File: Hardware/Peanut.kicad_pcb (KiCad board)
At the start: 2 copper layers, 96.8 x 57 mm, 54 parts, among them J1 Conn_02x04_Odd_Even, J2 Conn_02x04_Odd_Even, J3 AudioPlug3, SW1 Push_Button, SW2 Push_Button, SW3 Push_Button, SW4 Push_Button, SW5 Slide Switch, SW6 Slide Switch, U1 BNO085, U2 PCF8574, U3 HDC2010YPAR, U4 LTR-303ALS-01, U5 MCP4728T-E/UN, U6 LWP040-PSGLC-S, Y1 Crystal_32.768kHz

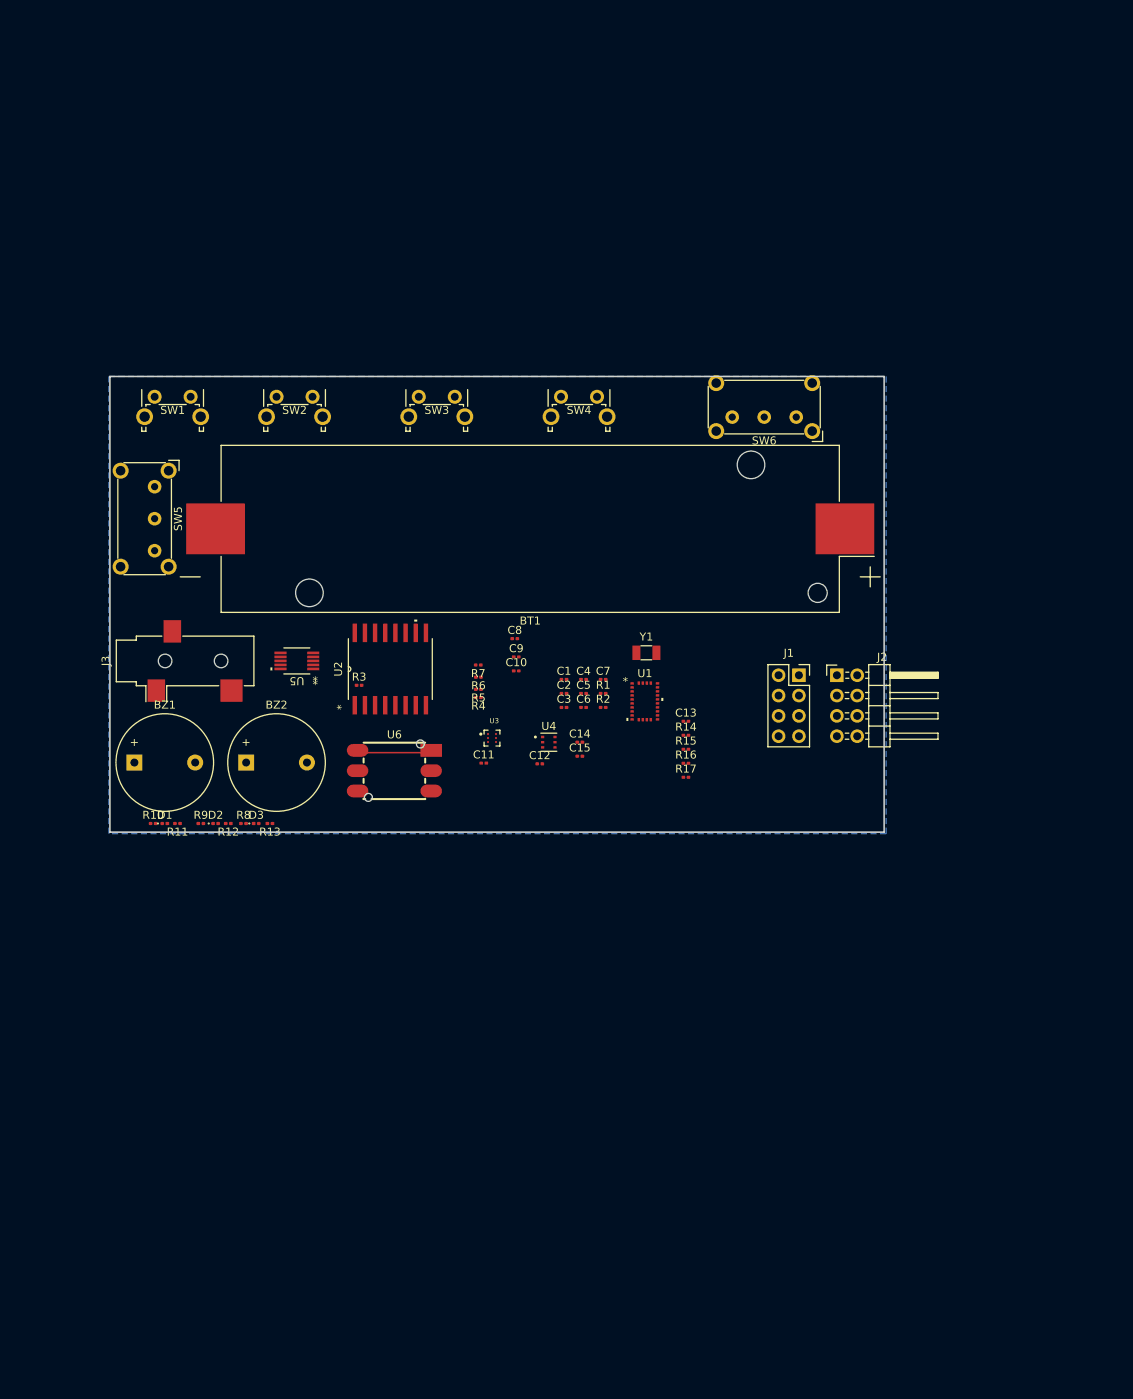
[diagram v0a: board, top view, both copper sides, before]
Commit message: Fully wired board!
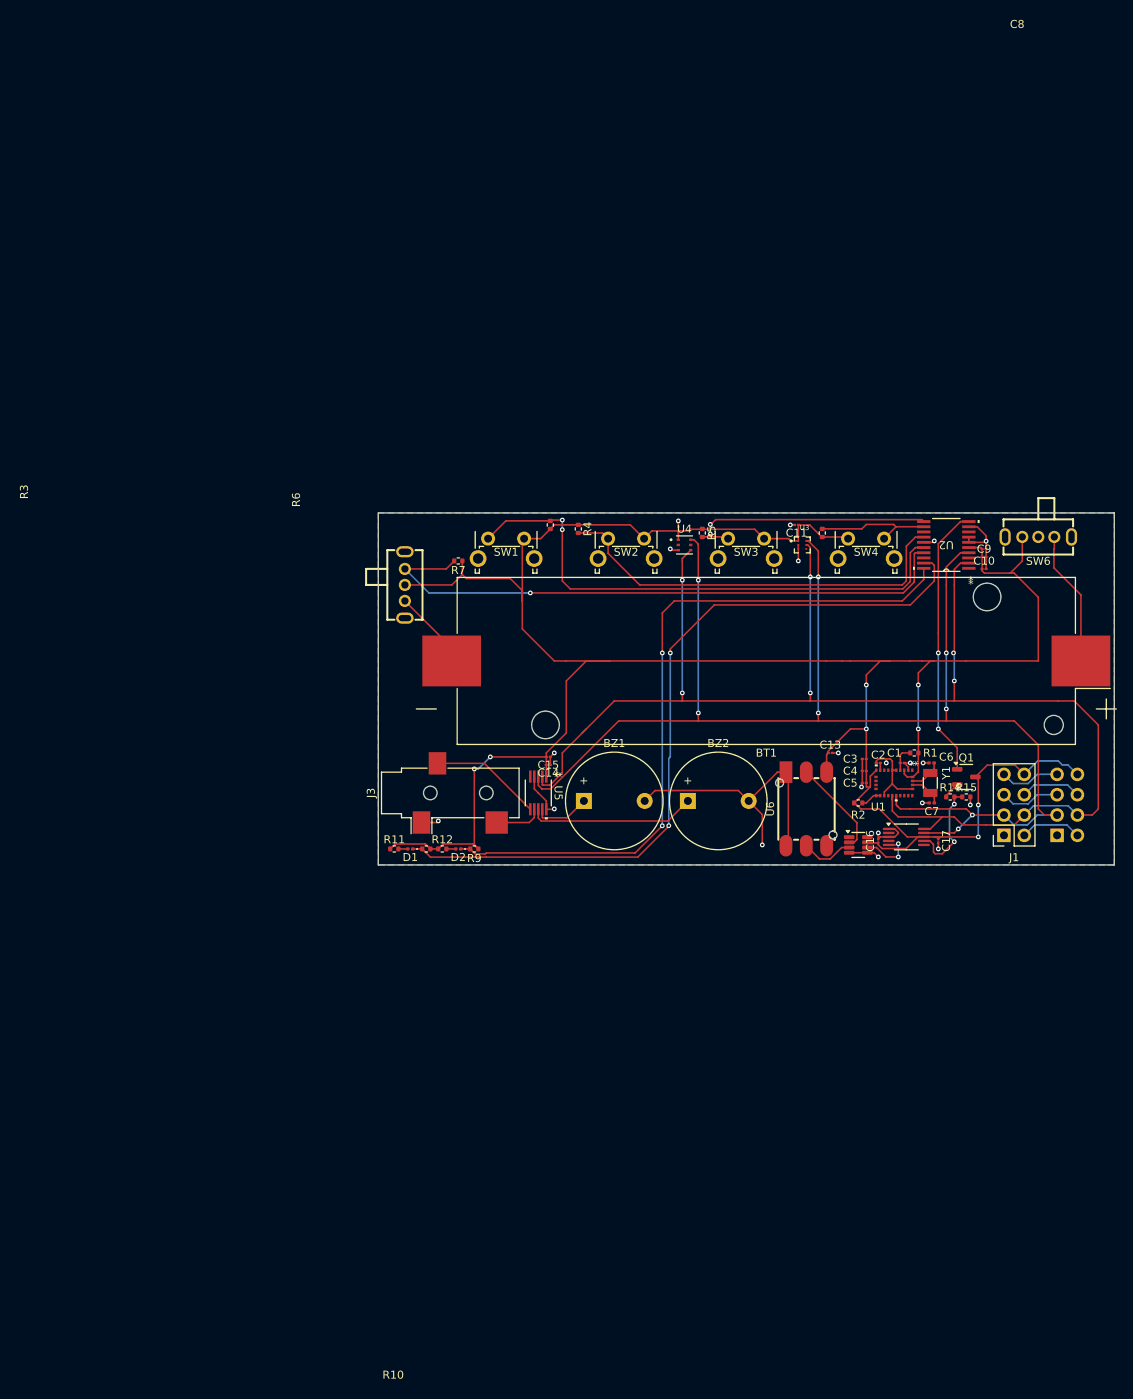
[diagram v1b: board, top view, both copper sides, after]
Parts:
- removed D3: BLU, LED_SMD:LED_0201_0603Metric
- removed R13: 2.2k, Resistor_SMD:R_0201_0603Metric
- removed R16, R17: 56k, Resistor_SMD:R_0201_0603Metric
- removed R8: 100k, Resistor_SMD:R_0201_0603Metric
- added C16: 0.1uF, Resistor_SMD:R_01005_0402Metric, F.Cu at (156.5, 86.0)
- added C17: 0.1uF, Resistor_SMD:R_01005_0402Metric, F.Cu at (164.0, 86.0)
- added Q1: Q_NPN_BEC, Package_TO_SOT_SMD:SOT-23-3, F.Cu at (167.5, 78.0)
- added U7: ADS1015IDGSR, Package_SO:VSSOP-10_3x3mm_P0.5mm, F.Cu at (160.0, 85.5)
- added U8: INA350ABSIDDFR, Package_TO_SOT_SMD:TSOT-23-8, F.Cu at (154.0, 86.5)
- C1, C10, C11, C12, C14, C15, C2, C3, C4, C5, C8, C9: footprint Capacitor_SMD:C_0201_0603Metric -> Resistor_SMD:R_01005_0402Metric
- C13: value 0.1uF -> 1uF; footprint Capacitor_SMD:C_0201_0603Metric -> Resistor_SMD:R_01005_0402Metric
- J2: footprint Connector_PinHeader_2.54mm:PinHeader_2x04_P2.54mm_Horizontal -> Peanut:PinHeader_2x04_P2.54mm_Horizontal_Flipped; moved to B.Cu
- R1, R10, R11, R12, R2, R3, R4, R5, R6, R7, R9: footprint Resistor_SMD:R_0201_0603Metric -> Resistor_SMD:R_0402_1005Metric
- R14, R15: value 1k -> R; footprint Resistor_SMD:R_0201_0603Metric -> Resistor_SMD:R_0402_1005Metric
- SW5, SW6: footprint Button_Switch_THT:SW_E-Switch_EG1224_SPDT_Angled -> Peanut:SW-TH_SK12D07VG4
- U2: value PCF8574 -> PCF8574APWR; footprint Peanut:DW16 -> Peanut:PW20
- moved U2 71.2 mm to (165.0, 49.0), turned to 180 degrees
- moved C10 59.8 mm to (169.7, 52.0)
- moved C9 59.8 mm to (169.7, 50.5)
- moved C8 59.7 mm to (169.7, 49.5)
- moved BZ1 56.4 mm to (119.7, 81.0)
- moved BZ2 55.4 mm to (132.7, 81.0)
- moved U6 51.7 mm to (147.5, 82.0), turned to 90 degrees
- moved C11 49.1 mm to (146.3, 46.5), turned to 180 degrees
- moved R6 46.6 mm to (149.5, 47.5), turned to 90 degrees
- moved U3 45.7 mm to (147.0, 49.0)
- moved SW1 45.3 mm to (107.7, 48.2)
- moved SW2 45.1 mm to (122.7, 48.2)
- moved C6 44.0 mm to (163.2, 76.2), turned to 180 degrees
- moved C7 43.9 mm to (163.2, 81.2), turned to 180 degrees
- moved C1 43.6 mm to (159.5, 76.2)
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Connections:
- C13 pad 1: GND -> +3V3
- C13 pad 2: /Pressure and ADC/PRESSURE -> GND
- R14 pad 1: Net-(U6-VOUT+) -> Net-(Q1-E)
- R14 pad 2: Net-(U7--) -> Net-(U7-AIN3)
- R15 pad 1: Net-(U7-+) -> Net-(U7-AIN3)
- R15 pad 2: Net-(U6-VOUT-) -> GND
- R3 pad 2: Net-(U2-P3) -> Net-(U2-P4)
- R4 pad 2: Net-(U2-P4) -> Net-(U2-P3)
- R5 pad 2: Net-(U2-P5) -> Net-(U2-P1)
- R6 pad 2: Net-(U2-P6) -> Net-(U2-P2)
- R7 pad 2: Net-(U2-P7) -> Net-(U2-P5)
- SW1 pad 1: Net-(U2-P3) -> Net-(U2-P4)
- SW2 pad 1: Net-(U2-P4) -> Net-(U2-P3)
- SW3 pad 1: Net-(U2-P5) -> Net-(U2-P1)
- SW4 pad 1: Net-(U2-P6) -> +3V3
- SW4 pad 2: +3V3 -> Net-(U2-P2)
- SW5 pad 1: Net-(U2-P7) -> Net-(U2-P5)
- U1 pad 17: /Motion Sensor/I2CADDR -> GND
- U2 pad 1: GND -> /DigitalMuxer/~{INT}
- U2 pad 10: Net-(U2-P5) -> /DigitalMuxer/P2
- U2 pad 11: Net-(U2-P6) -> Net-(U2-P1)
- U2 pad 12: Net-(U2-P7) -> Net-(U2-P2)
- U2 pad 13: /DigitalMuxer/Reset pin -> unconnected-(U2-NC-Pad13)
- U2 pad 14: SCL -> Net-(U2-P3)
- U2 pad 15: SDA -> GND
- U2 pad 16: +3V3 -> Net-(U2-P4)
- U2 pad 2: GND -> SCL
- U2 pad 3: GND -> unconnected-(U2-NC-Pad3)
- U2 pad 4: Net-(D1-K) -> SDA
- U2 pad 5: Net-(D2-K) -> +3V3
- U2 pad 6: Net-(D3-K) -> GND
- U2 pad 7: Net-(U2-P3) -> GND
- U2 pad 8: GND -> unconnected-(U2-NC-Pad8)
- U2 pad 9: Net-(U2-P4) -> GND
- U5 pad 5: unconnected-(U5-RDY/~{BSY}-Pad5) -> /DAC and Sound/RDY/~{BSY}
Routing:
- net +3V3: track 0.00 -> 320.3 mm, vias 0 -> 8
- net SCL: track 0.00 -> 180.2 mm, vias 0 -> 6
- net SDA: track 0.00 -> 179.0 mm, vias 0 -> 8
- net Net-(D1-K): track 0.00 -> 96.1 mm, vias 0 -> 2
- net GND: track 9.63 -> 100.2 mm, vias 0 -> 20
- net Net-(D2-K): track 0.00 -> 89.3 mm, vias 0 -> 2
- net Net-(U2-P5): track 0.00 -> 76.8 mm, vias 0 -> 1
- net Net-(U2-P4): track 0.00 -> 67.7 mm, vias 0 -> 2
- net Net-(U2-P3): track 0.00 -> 52.0 mm
- net /DigitalMuxer/P2: track 0.00 -> 34.1 mm, vias 0 -> 2
- net Net-(U2-P1): track 0.00 -> 31.9 mm, vias 0 -> 2
- net Net-(BZ2-+): track 0.00 -> 21.0 mm
- net Net-(BT1-+): track 0.00 -> 16.9 mm
- net Net-(U2-P2): track 0.00 -> 14.7 mm
- net Net-(U5-VOUTA): track 0.00 -> 14.0 mm
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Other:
- board size 96.8 x 57 mm -> 92 x 44 mm
